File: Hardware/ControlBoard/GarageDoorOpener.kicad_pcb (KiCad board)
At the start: 2 copper layers, 48 parts, among them J1 Conn_01x04, J2 RJ45, Q1 DMG1012T-7, U1 Argon/Boron, U2 TPS56637, U3 CPC1002N, U4 VL53L1X

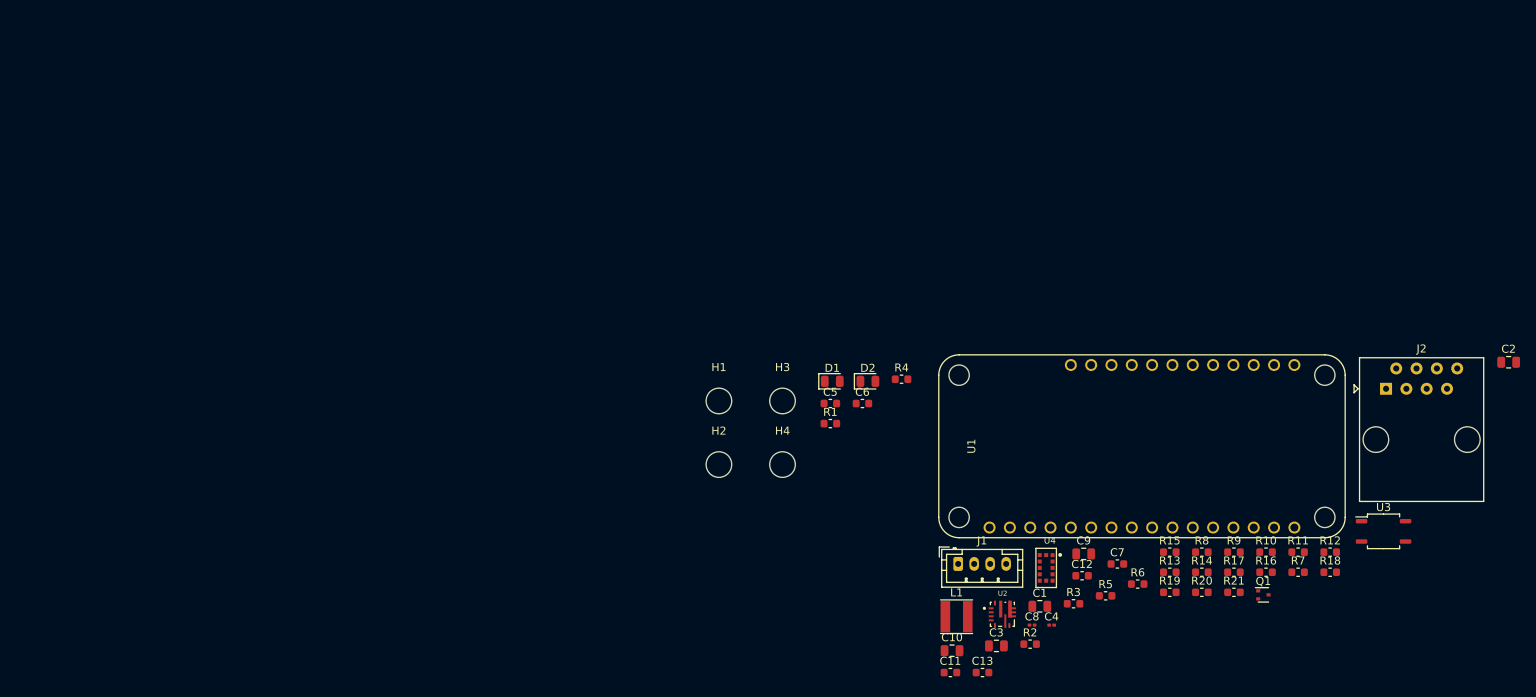
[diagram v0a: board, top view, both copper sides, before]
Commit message: working on the PCB for the control board
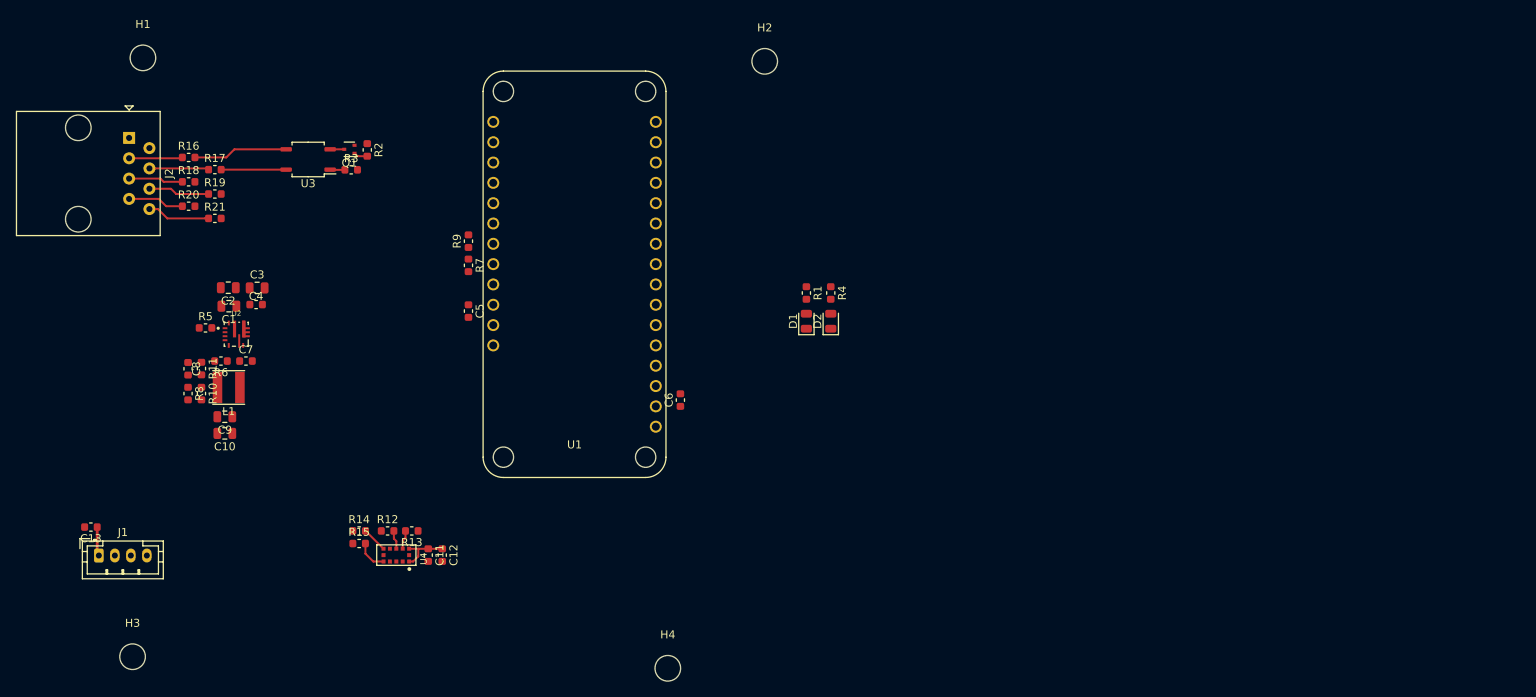
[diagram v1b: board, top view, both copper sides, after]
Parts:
- C4, C8: footprint Capacitor_SMD:C_0201_0603Metric -> Capacitor_SMD:C_0603_1608Metric
- moved C2 160.3 mm to (110.6, 85.6), turned to 180 degrees
- moved J2 160.2 mm to (98.2, 66.9), turned to 270 degrees
- moved R18 150.8 mm to (105.7, 72.4)
- moved R16 144.3 mm to (105.7, 69.3)
- moved U3 142.2 mm to (120.6, 69.6), turned to 180 degrees
- moved R11 139.0 mm to (107.3, 95.7), turned to 270 degrees
- moved R17 137.0 mm to (108.9, 70.9)
- moved R21 135.7 mm to (108.9, 77.0)
- moved R20 135.5 mm to (105.7, 75.4)
- moved R10 134.5 mm to (107.3, 98.9), turned to 270 degrees
- moved R19 129.3 mm to (108.9, 73.9)
- moved R8 128.3 mm to (105.6, 98.9), turned to 270 degrees
- moved Q1 127.1 mm to (125.8, 68.3), turned to 180 degrees
- moved R6 117.9 mm to (109.7, 94.8), turned to 180 degrees
- moved R12 117.9 mm to (130.5, 116.0)
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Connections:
- U3 pad 3: /Relay_Ouput2 -> /Relay_Ouput1
- U3 pad 4: /Relay_Ouput1 -> /Relay_Ouput2
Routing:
- net /Relay_Ouput1: track 0.00 -> 11.8 mm
- net /Relay_Ouput2: track 0.00 -> 8.12 mm
- net Net-(J2-Pad8): track 0.00 -> 7.88 mm
- net Net-(J2-Pad6): track 0.00 -> 7.66 mm
- net Net-(J2-Pad4): track 0.00 -> 7.45 mm
- net Net-(J2-Pad7): track 0.00 -> 7.03 mm
- net Net-(J2-Pad5): track 0.00 -> 6.82 mm
- net Net-(J2-Pad3): track 0.00 -> 6.70 mm
- net +3V3: track 0.00 -> 6.50 mm
- net /SENSOR_SHUTDOWN: track 0.00 -> 3.94 mm
- net +5V: track 0.00 -> 3.64 mm
- net /SENSOR_INT: track 0.00 -> 3.18 mm
- net /SENSOR_I2C_SCL: track 0.00 -> 2.36 mm
- net /SENSOR_I2C_SDA: track 0.00 -> 2.35 mm
- net Net-(R3-Pad1): track 0.00 -> 1.86 mm
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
